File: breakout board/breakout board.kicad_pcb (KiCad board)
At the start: 2 copper layers, 3 parts, among them J1 Conn_01x07_Pin, J2 Conn_01x07_Pin, U1 MCP2518FD-xQBB

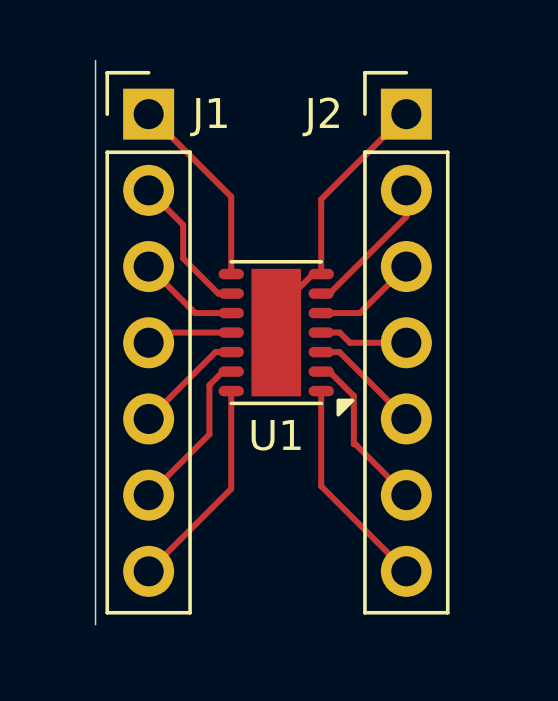
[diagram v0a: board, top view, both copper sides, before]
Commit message: where are you
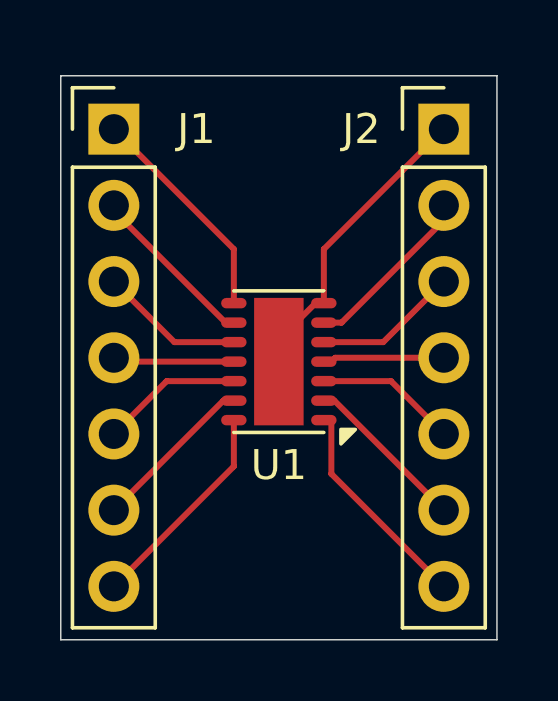
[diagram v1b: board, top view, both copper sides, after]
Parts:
- moved J2 1.35 mm to (131.8, 97.0)
- moved J1 1.26 mm to (120.8, 97.0)
- moved U1 0.97 mm to (126.2, 104.8)
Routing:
- net Net-(J1-Pin_3): track 3.40 -> 4.84 mm
- net Net-(J2-Pin_3): track 3.48 -> 4.84 mm
- net Net-(J1-Pin_4): track 2.89 -> 4.05 mm
- net Net-(J2-Pin_2): track 4.78 -> 5.91 mm
- net Net-(J2-Pin_4): track 2.98 -> 4.05 mm
- net Net-(J1-Pin_5): track 3.68 -> 4.73 mm
- net Net-(J1-Pin_1): track 6.47 -> 7.46 mm
- net Net-(J2-Pin_5): track 3.76 -> 4.73 mm
- net Net-(J2-Pin_1): track 9.24 -> 10.2 mm
- net Net-(J1-Pin_2): track 4.83 -> 5.73 mm
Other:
- board outline added: 14.5 x 18.8 mm
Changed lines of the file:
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@@
 	(footprint "Connector_PinHeader_2.54mm:PinHeader_1x07_P2.54mm_Vertical"
 		(layer "F.Cu")
-		(at 130.5 96.5)
+		(at 131.75 97)
 		(descr "Through hole straight pin header, 1x07, 2.54mm pitch, single row")
 		(tags "Through hole pin header THT 1x07 2.54mm single row")
@@
 			(at 0 17.62 0)
 			(layer "F.Fab")
+			(hide yes)
 			(effects
 				(font
@@
 	(footprint "Package_DFN_QFN:DFN-14-1EP_3x4.5mm_P0.65mm_EP1.65x4.25mm"
 		(layer "F.Cu")
-		(at 126.1625 103.78125 180)
+		(at 126.25 104.75 180)
 		(descr "14-lead very thin plastic quad flat, 3.0x4.5mm size, 0.65mm pitch (http://ww1.microchip.com/downloads/en/DeviceDoc/14L_VDFN_4_5x3_0mm_JHA_C041198A.pdf)")
 		(tags "VDFN DFN 0.65mm")
@@
 			)
 			(layer "F.Fab")
-		)
-		(fp_text user "${REFERENCE}"
-			(at 0 2.25 90)
-			(layer "F.Fab")
-			(effects
-				(font
-					(size 0.8 0.8)
-					(thickness 0.12)
-				)
-			)
 		)
 		(pad "" smd rect
@@
 	(footprint "Connector_PinHeader_2.54mm:PinHeader_1x07_P2.54mm_Vertical"
 		(layer "F.Cu")
-		(at 121.91 96.5)
+		(at 120.75 97)
 		(descr "Through hole straight pin header, 1x07, 2.54mm pitch, single row")
 		(tags "Through hole pin header THT 1x07 2.54mm single row")
 		(property "Reference" "J1"
-			(at 2.09 0 0)
+			(at 2.75 0 0)
 			(layer "F.SilkS")
 			(effects
@@
 	)
 	(gr_line
-		(start 120.14 113.52)
-		(end 120.14 94.72)
+		(start 133.52 95.22)
+		(end 133.52 114.02)
 		(stroke
 			(width 0.05)
@@
 		(layer "Edge.Cuts")
 	)
-	(segment
-		(start 124.6625 101.83125)
-		(end 124.6625 99.2525)
+	(gr_line
+		(start 118.98 95.22)
+		(end 133.52 95.22)
+		(stroke
+			(width 0.05)
+			(type default)
+		)
+		(layer "Edge.Cuts")
+	)
+	(gr_line
+		(start 133.52 114.02)
+		(end 118.98 114.02)
+		(stroke
+			(width 0.05)
+			(type default)
+		)
+		(layer "Edge.Cuts")
+	)
+	(gr_line
+		(start 118.98 114.02)
+		(end 118.98 95.22)
+		(stroke
+			(width 0.05)
+			(type default)
+		)
+		(layer "Edge.Cuts")
+	)
+	(segment
+		(start 124.75 101)
+		(end 120.75 97)
 		(width 0.2)
 		(layer "F.Cu")
@@
 	)
 	(segment
-		(start 124.6625 99.2525)
-		(end 121.91 96.5)
+		(start 124.75 102.8)
+		(end 124.75 101)
 		(width 0.2)
 		(layer "F.Cu")
@@
 	)
 	(segment
-		(start 124.389334 105.08125)
-		(end 123.9365 105.534084)
+		(start 124.75 106.05)
+		(end 124.4 106.05)
 		(width 0.2)
 		(layer "F.Cu")
@@
 	)
 	(segment
-		(start 123.9365 105.534084)
-		(end 123.9365 107.1735)
+		(start 124.4 106.05)
+		(end 120.75 109.7)
 		(width 0.2)
 		(layer "F.Cu")
@@
 	)
 	(segment
-		(start 123.9365 107.1735)
-		(end 121.91 109.2)
-		(width 0.2)
-		(layer "F.Cu")
-		(net 2)
-	)
-	(segment
-		(start 124.6625 105.08125)
-		(end 124.389334 105.08125)
-		(width 0.2)
-		(layer "F.Cu")
-		(net 2)
-	)
-	(segment
-		(start 122.24875 103.78125)
-		(end 121.91 104.12)
+		(start 120.88 104.75)
+		(end 120.75 104.62)
 		(width 0.2)
 		(layer "F.Cu")
@@
 	)
 	(segment
-		(start 124.6625 103.78125)
-		(end 122.24875 103.78125)
+		(start 124.75 104.75)
+		(end 120.88 104.75)
 		(width 0.2)
 		(layer "F.Cu")
@@
 	)
 	(segment
-		(start 124.6625 102.48125)
-		(end 124.23125 102.48125)
+		(start 124.75 103.45)
+		(end 124.475 103.45)
 		(width 0.2)
 		(layer "F.Cu")
@@
 	)
 	(segment
-		(start 123.061 100.191)
-		(end 121.91 99.04)
+		(start 120.75 99.725)
+		(end 120.75 99.54)
 		(width 0.2)
 		(layer "F.Cu")
@@
 	)
 	(segment
-		(start 124.23125 102.48125)
-		(end 123.061 101.311)
+		(start 124.475 103.45)
+		(end 120.75 99.725)
 		(width 0.2)
 		(layer "F.Cu")
@@
 	)
 	(segment
-		(start 123.061 101.311)
-		(end 123.061 100.191)
-		(width 0.2)
-		(layer "F.Cu")
-		(net 4)
-	)
-	(segment
-		(start 124.6625 104.43125)
-		(end 124.13875 104.43125)
+		(start 122.51 105.4)
+		(end 120.75 107.16)
 		(width 0.2)
 		(layer "F.Cu")
@@
 	)
 	(segment
-		(start 124.13875 104.43125)
-		(end 121.91 106.66)
+		(start 124.75 105.4)
+		(end 122.51 105.4)
 		(width 0.2)
 		(layer "F.Cu")
@@
 	)
 	(segment
-		(start 124.6625 103.13125)
-		(end 123.46125 103.13125)
+		(start 122.77 104.1)
+		(end 120.75 102.08)
 		(width 0.2)
 		(layer "F.Cu")
@@
 	)
 	(segment
-		(start 123.46125 103.13125)
-		(end 121.91 101.58)
+		(start 124.75 104.1)
+		(end 122.77 104.1)
 		(width 0.2)
 		(layer "F.Cu")
@@
 	)
 	(segment
-		(start 124.6625 108.9875)
-		(end 121.91 111.74)
+		(start 124.75 106.7)
+		(end 124.75 108.24)
 		(width 0.2)
 		(layer "F.Cu")
@@
 	)
 	(segment
-		(start 124.6625 105.73125)
-		(end 124.6625 108.9875)
+		(start 124.75 108.24)
+		(end 120.75 112.24)
 		(width 0.2)
 		(layer "F.Cu")
@@
 	)
 	(segment
-		(start 128.94875 103.13125)
-		(end 130.5 101.58)
+		(start 129.73 104.1)
+		(end 131.75 102.08)
 		(width 0.2)
 		(layer "F.Cu")
@@
 	)
 	(segment
-		(start 127.6625 103.13125)
-		(end 128.94875 103.13125)
+		(start 127.75 104.1)
+		(end 129.73 104.1)
 		(width 0.2)
 		(layer "F.Cu")
@@
 	)
 	(segment
-		(start 127.6625 104.43125)
-		(end 128.27125 104.43125)
+		(start 129.99 105.4)
+		(end 131.75 107.16)
 		(width 0.2)
 		(layer "F.Cu")
@@
 	)
 	(segment
-		(start 128.27125 104.43125)
-		(end 130.5 106.66)
+		(start 127.75 105.4)
+		(end 129.99 105.4)
 		(width 0.2)
 		(layer "F.Cu")
@@
 	)
 	(segment
-		(start 127.6625 102.48125)
-		(end 127.9375 102.48125)
+		(start 131.75 100.04)
+		(end 131.75 99.54)
 		(width 0.2)
 		(layer "F.Cu")
@@
 	)
 	(segment
-		(start 130.5 99.91875)
-		(end 130.5 99.04)
+		(start 128.34 103.45)
+		(end 131.75 100.04)
 		(width 0.2)
 		(layer "F.Cu")
@@
 	)
 	(segment
-		(start 127.9375 102.48125)
-		(end 130.5 99.91875)
+		(start 127.75 103.45)
+		(end 128.34 103.45)
 		(width 0.2)
 		(layer "F.Cu")
@@
 	)
 	(segment
-		(start 127.6625 105.73125)
-		(end 127.6625 108.9025)
+		(start 127.75 106.7)
+		(end 127.95 106.7)
 		(width 0.2)
 		(layer "F.Cu")
@@
 	)
 	(segment
-		(start 127.6625 108.9025)
-		(end 130.5 111.74)
+		(start 128 108.49)
+		(end 131.75 112.24)
 		(width 0.2)
 		(layer "F.Cu")
@@
 	)
 	(segment
-		(start 126.1625 103.05625)
-		(end 126.1625 103.78125)
+		(start 127.95 106.7)
+		(end 128 106.75)
+		(width 0.2)
+		(layer "F.Cu")
+		(net 11)
+	)
+	(segment
+		(start 128 106.75)
+		(end 128 108.49)
+		(width 0.2)
+		(layer "F.Cu")
+		(net 11)
+	)
+	(segment
+		(start 127.75 101)
+		(end 131.75 97)
 		(width 0.2)
 		(layer "F.Cu")
@@
 	)
 	(segment
-		(start 127.6625 101.83125)
-		(end 127.3875 101.83125)
+		(start 127.475 102.8)
+		(end 126.25 104.025)
 		(width 0.2)
 		(layer "F.Cu")
@@
 	)
 	(segment
-		(start 127.6625 101.83125)
-		(end 127.6625 99.3375)
+		(start 126.25 104.025)
+		(end 126.25 104.75)
 		(width 0.2)
 		(layer "F.Cu")
@@
 	)
 	(segment
-		(start 127.3875 101.83125)
-		(end 126.1625 103.05625)
+		(start 127.75 102.8)
+		(end 127.475 102.8)
 		(width 0.2)
 		(layer "F.Cu")
@@
 	)
 	(segment
-		(start 127.6625 99.3375)
-		(end 130.5 96.5)
+		(start 127.75 102.8)
+		(end 127.75 101)
 		(width 0.2)
 		(layer "F.Cu")
@@
 	)
 	(segment
-		(start 127.6625 103.78125)
-		(end 128.28125 103.78125)
+		(start 128.13 104.62)
+		(end 131.75 104.62)
 		(width 0.2)
 		(layer "F.Cu")
@@
 	)
 	(segment
-		(start 128.62 104.12)
-		(end 130.5 104.12)
+		(start 127.75 104.75)
+		(end 128 104.75)
 		(width 0.2)
 		(layer "F.Cu")
@@
 	)
 	(segment
-		(start 128.28125 103.78125)
-		(end 128.62 104.12)
+		(start 128 104.75)
+		(end 128.13 104.62)
 		(width 0.2)
 		(layer "F.Cu")
@@
 	)
 	(segment
-		(start 128.75 105.895584)
-		(end 128.75 107.5)
+		(start 128.1 106.05)
+		(end 131.75 109.7)
 		(width 0.2)
 		(layer "F.Cu")
@@
 	)
 	(segment
-		(start 128.8 107.5)
-		(end 130.5 109.2)
-		(width 0.2)
-		(layer "F.Cu")
-		(net 14)
-	)
-	(segment
-		(start 127.6625 105.08125)
-		(end 127.935666 105.08125)
-		(width 0.2)
-		(layer "F.Cu")
-		(net 14)
-	)
-	(segment
-		(start 128.75 107.5)
-		(end 128.8 107.5)
-		(width 0.2)
-		(layer "F.Cu")
-		(net 14)
-	)
-	(segment
-		(start 127.935666 105.08125)
-		(end 128.75 105.895584)
-		(width 0.2)
-		(layer "F.Cu")
+		(start 127.75 106.05)
+		(end 128.1 106.05)
+		(width 0.2)
+		(layer "F.Cu")
